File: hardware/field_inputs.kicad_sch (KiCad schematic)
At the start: 100 parts, among them J26 Dedicated START button input, J27 Expansion inputs 4-7; 1=GND, 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, J5 Dedicated E-stop loop, J6 Dedicated HOLD button input, J7 PLC positions 1-8; software-m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, J8 PLC positions 9-16; software-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, J9 Expansion inputs 0-3; 1=GND, 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, U18 LTV-847S, U19 LTV-847S, U20 LTV-847S, U21 LTV-847S, U35 EL3H7, U36 EL3H7, U39 EL3H7, U40 TBA2-0512

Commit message: Update RP2350B PCB, pinout and fabrication rules
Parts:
- removed J7: PLC positions 1-8; software-mapped isolated inputs, Connector_Phoenix_MC:PhoenixContact_MCV_1,5_16-G-3.5_1x16_P3.50mm_Vertical, symbol Connector_Generic:Conn_01x16
- removed J8: PLC positions 9-16; software-mapped isolated inpu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, Connector_Phoenix_MC:PhoenixContact_MCV_1,5_16-G-3.5_1x16_P3.50mm_Vertical, symbol Connector_Generic:Conn_01x16
- added J34: PLC positions 5-8 of J7 bank; software-mapped iso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, Connector_Phoenix_MC:PhoenixContact_MCV_1,5_8-G-3.5_1x08_P3.50mm_Vertical, symbol Connector_Generic:Conn_01x08
- added J35: PLC positions 5-8 of J8 bank; software-mapped iso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, Connector_Phoenix_MC:PhoenixContact_MCV_1,5_8-G-3.5_1x08_P3.50mm_Vertical, symbol Connector_Generic:Conn_01x08
- added J7: PLC positions 1-4; software-mapped isolated inputs, Connector_Phoenix_MC:PhoenixContact_MCV_1,5_8-G-3.5_1x08_P3.50mm_Vertical, symbol Connector_Generic:Conn_01x08
- added J8: PLC positions 9-12; software-mapped isolated inpu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, Connector_Phoenix_MC:PhoenixContact_MCV_1,5_8-G-3.5_1x08_P3.50mm_Vertical, symbol Connector_Generic:Conn_01x08
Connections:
- net FIELD_COM0: now also J34.2 (Pin_2), J34.4 (Pin_4), J34.6 (Pin_6), J34.8 (Pin_8), J7.2 (Pin_2), J7.4 (Pin_4), J7.6 (Pin_6), J7.8 (Pin_8)
- net FIELD_COM1: now also J35.2 (Pin_2), J35.4 (Pin_4), J35.6 (Pin_6), J35.8 (Pin_8), J8.2 (Pin_2), J8.4 (Pin_4), J8.6 (Pin_6), J8.8 (Pin_8)
- net FIELD_IN1: now also J8.1 (Pin_1)
- net FIELD_IN10: now also J7.3 (Pin_3)
- net FIELD_IN11: now also J7.5 (Pin_5)
- net FIELD_IN12: now also J7.7 (Pin_7)
- net FIELD_IN13: now also J34.1 (Pin_1)
- net FIELD_IN14: now also J34.3 (Pin_3)
- net FIELD_IN15: now also J34.5 (Pin_5)
- net FIELD_IN16: now also J34.7 (Pin_7)
- net FIELD_IN2: now also J8.3 (Pin_3)
- net FIELD_IN3: now also J8.5 (Pin_5)
- net FIELD_IN4: now also J8.7 (Pin_7)
- net FIELD_IN5: now also J35.1 (Pin_1)
- net FIELD_IN6: now also J35.3 (Pin_3)
- net FIELD_IN7: now also J35.5 (Pin_5)
- net FIELD_IN8: now also J35.7 (Pin_7)
- net FIELD_IN9: now also J7.1 (Pin_1)

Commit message: Update RP2350 board power and I/O design
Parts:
- removed R76, R77, R78, R79, R80, R81, R82, R83, R84, R85, R86, R87, R88, R89, R90, R91: 4.7k, Resistor_SMD:R_1206_3216Metric, symbol Device:R
- added RN32, RN33, RN34, RN35: 4x4.7k, Resistor_SMD:R_Array_Convex_4x0603, symbol LeanCam:ResistorPack04
- C103: value 10uF -> 22uF 25V; footprint Capacitor_SMD:C_1206_3216Metric -> Capacitor_SMD:C_1210_3225Metric; MPN CL31 series 1206 X7R 10uF -> CL32 series 1210 X7R 22uF 25V
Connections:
- net +3V3: now also RN32.5 (R4B), RN32.6 (R3B), RN32.7 (R2B), RN32.8 (R1B), RN33.5 (R4B), RN33.6 (R3B), RN33.7 (R2B), RN33.8 (R1B), RN34.5 (R4B), RN34.6 (R3B), RN34.7 (R2B), RN34.8 (R1B), RN35.5 (R4B), RN35.6 (R3B), RN35.7 (R2B), RN35.8 (R1B)
- net PLC_IN10_N: now also RN34.2 (R2A)
- net PLC_IN11_N: now also RN34.3 (R3A)
- net PLC_IN12_N: now also RN34.4 (R4A)
- net PLC_IN13_N: now also RN35.1 (R1A)
- net PLC_IN14_N: now also RN35.2 (R2A)
- net PLC_IN15_N: now also RN35.3 (R3A)
- net PLC_IN16_N: now also RN35.4 (R4A)
- net PLC_IN1_N: now also RN32.1 (R1A)
- net PLC_IN2_N: now also RN32.2 (R2A)
- net PLC_IN3_N: now also RN32.3 (R3A)
- net PLC_IN4_N: now also RN32.4 (R4A)
- net PLC_IN5_N: now also RN33.1 (R1A)
- net PLC_IN6_N: now also RN33.2 (R2A)
- net PLC_IN7_N: now also RN33.3 (R3A)
- net PLC_IN8_N: now also RN33.4 (R4A)
- net PLC_IN9_N: now also RN34.1 (R1A)

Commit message: Standardize passives and add microSD alternate
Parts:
- C103: value 22uF 25V -> 22uF 50V; MPN CL32 series 1210 X7R 22uF 25V -> CL32 series 1210 X7R 22uF 50V
- RN32, RN33, RN34, RN35: value 4x4.7k -> 4x10k; MPN YC164-FR-074K7L -> YC164-FR-0710KL

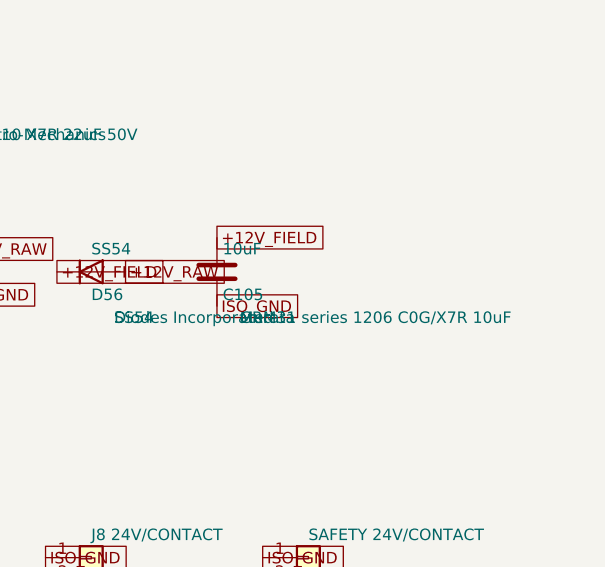
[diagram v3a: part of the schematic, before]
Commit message: BOM simplification
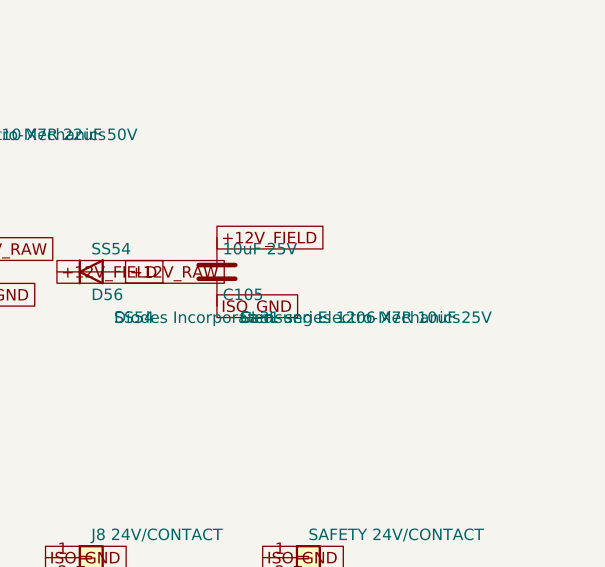
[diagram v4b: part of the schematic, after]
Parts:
- C105: value 10uF -> 10uF 25V; MPN GRM31 series 1206 C0G/X7R 10uF -> CL31 series 1206 X7R 10uF 25V; Manufacturer Murata -> Samsung Electro-Mechanics
